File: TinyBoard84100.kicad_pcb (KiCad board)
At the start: 2 copper layers, 28.2 x 15.2 mm, 14 parts, among them P1 CONN_01X02, P2 CONN_01X07, P3 CONN_01X07, P4 CONN_02X03, SW1 SW_PUSH, U1 78L05, U2 ATTINY841

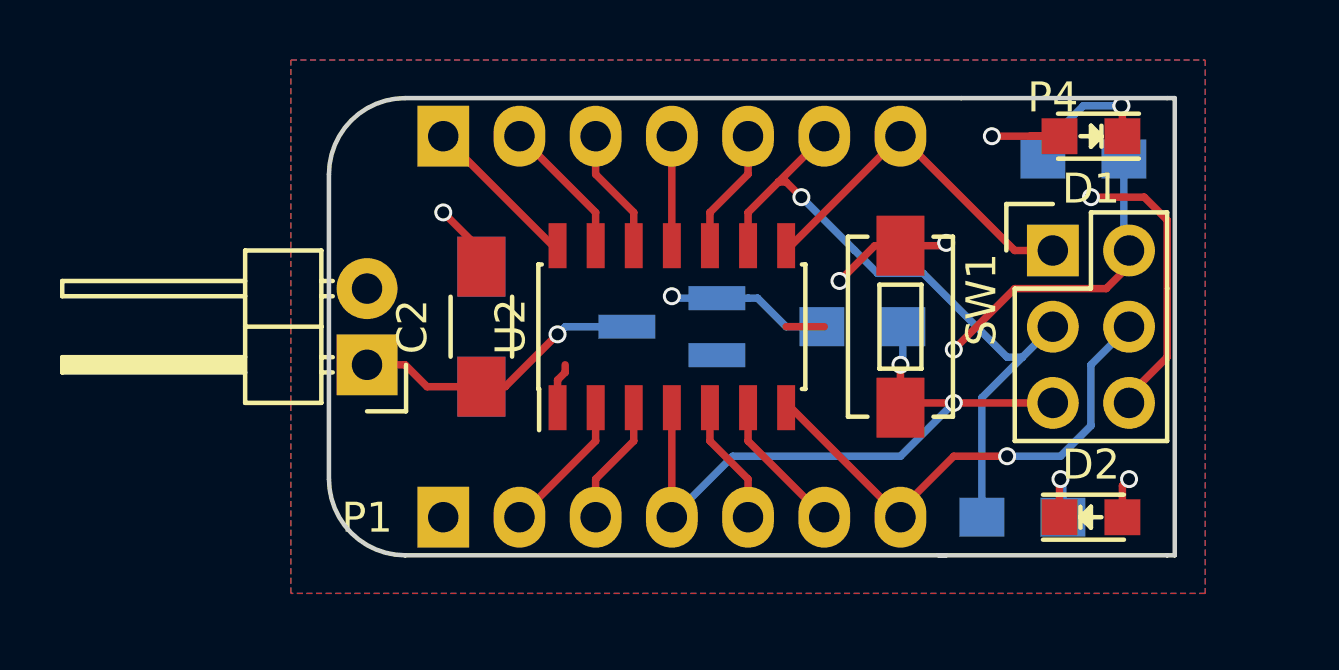
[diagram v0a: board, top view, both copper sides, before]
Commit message: gerbers
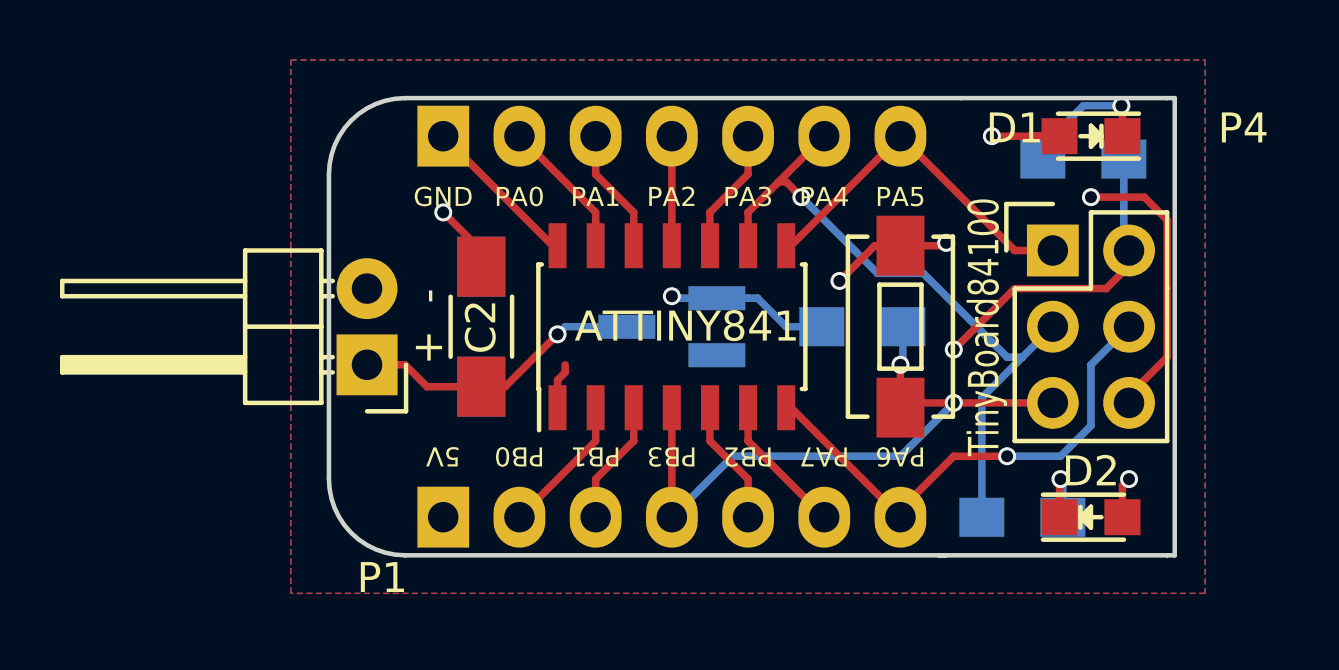
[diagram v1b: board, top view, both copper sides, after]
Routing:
- net (no net): track 1.27 -> 0.00 mm
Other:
- board text added: "+ -"
- board text added: "5V"
- board text added: "GND"
- board text added: "PA0"
- board text added: "PA1"
- board text added: "PA2"
- board text added: "PA3"
- board text added: "PA4"
- board text added: "PA5"
- board text added: "PA6"
- board text added: "PA7"
- board text added: "PB0"
- board text added: "PB1"
- board text added: "PB2"
- board text added: "PB3"
- board text added: "TinyBoard84100"
